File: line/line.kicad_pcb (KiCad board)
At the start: 2 copper layers, 60 x 80 mm, 42 parts, among them J1 MAINS, J2 CONTROL, Q1 WMM38N60C2, Q2 WMM38N60C2, U1 LM324, U2 LTV-817S

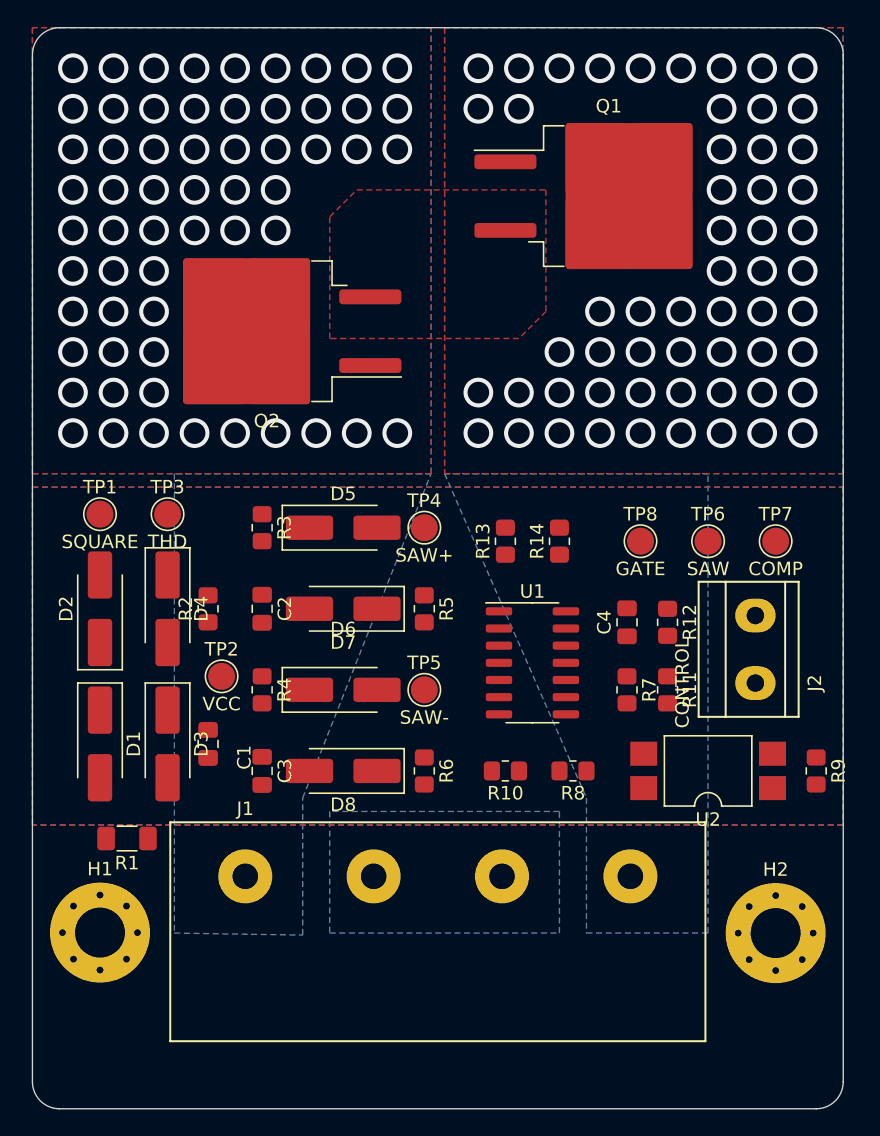
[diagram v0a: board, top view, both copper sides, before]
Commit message: WIP
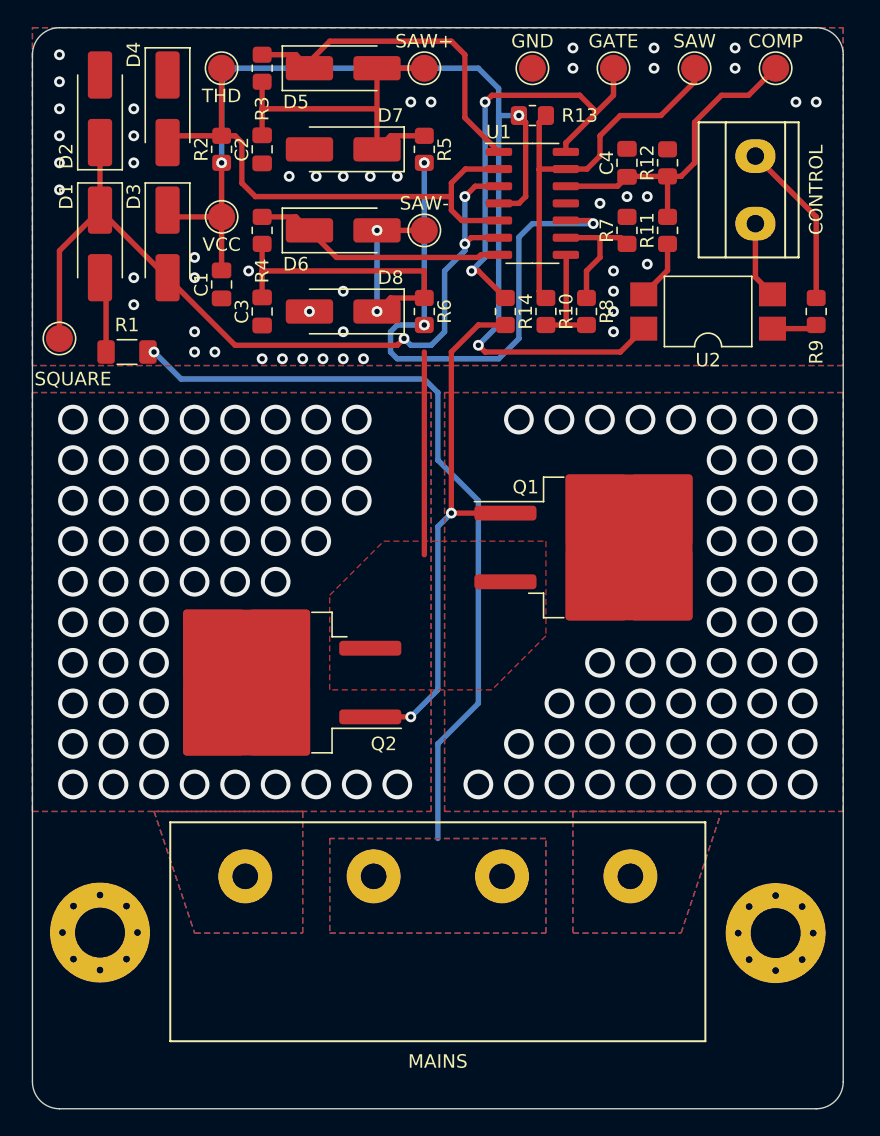
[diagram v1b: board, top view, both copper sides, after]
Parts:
- added TP9: GND, TestPoint:TestPoint_Pad_D2.0mm, F.Cu at (137.0, 73.0)
- moved D1 37.0 mm to (105.0, 86.0)
- moved D2 37.0 mm to (105.0, 76.0)
- moved D3 37.0 mm to (110.0, 86.0)
- moved D4 37.0 mm to (110.0, 76.0)
- moved R1 36.0 mm to (107.0, 94.0)
- moved TP8 35.1 mm to (143.0, 73.0)
- moved TP6 35.0 mm to (149.0, 73.0)
- moved TP7 35.0 mm to (155.0, 73.0)
- moved R10 34.1 mm to (138.0, 91.0), turned to 90 degrees
- moved C1 34.0 mm to (114.0, 89.0)
- moved R2 34.0 mm to (114.0, 79.0)
- moved R8 34.0 mm to (141.0, 91.0), turned to -90 degrees
- moved C2 34.0 mm to (117.0, 79.0)
- moved C3 34.0 mm to (117.0, 91.0)
- moved C4 34.0 mm to (144.0, 80.0)
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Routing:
- net VCC: track 0.00 -> 83.9 mm, vias 0 -> 3
- net Net-(D1-K): track 0.00 -> 62.4 mm, vias 0 -> 3
- net /MAINS_N: track 0.00 -> 58.2 mm, vias 0 -> 1
- net Net-(U1C-+): track 0.00 -> 42.1 mm, vias 0 -> 3
- net Net-(Q1-G): track 0.00 -> 40.1 mm, vias 0 -> 2
- net Net-(D4-A): track 0.00 -> 39.6 mm
- net Net-(R14-Pad1): track 0.00 -> 32.9 mm, vias 0 -> 2
- net Net-(D6-A): track 0.00 -> 31.4 mm, vias 0 -> 2
- net Net-(U1D--): track 0.00 -> 30.0 mm
- net Net-(D5-A): track 0.00 -> 25.9 mm
- net Net-(D5-K): track 0.00 -> 25.2 mm
- net Net-(U1D-+): track 0.00 -> 23.9 mm
- net Net-(D6-K): track 0.00 -> 18.8 mm
- net GND: track 0.00 -> 15.0 mm, vias 0 -> 49
- net Net-(J2-Pin_2): track 0.00 -> 12.4 mm
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- added copper zone on F.Cu, net /MAINS_N
